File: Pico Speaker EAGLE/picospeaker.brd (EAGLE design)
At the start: 77.1 x 76.2 mm, 9 parts, among them J1 SPK -/+ MAX 3W, J2 POWER -/+ 4,5v

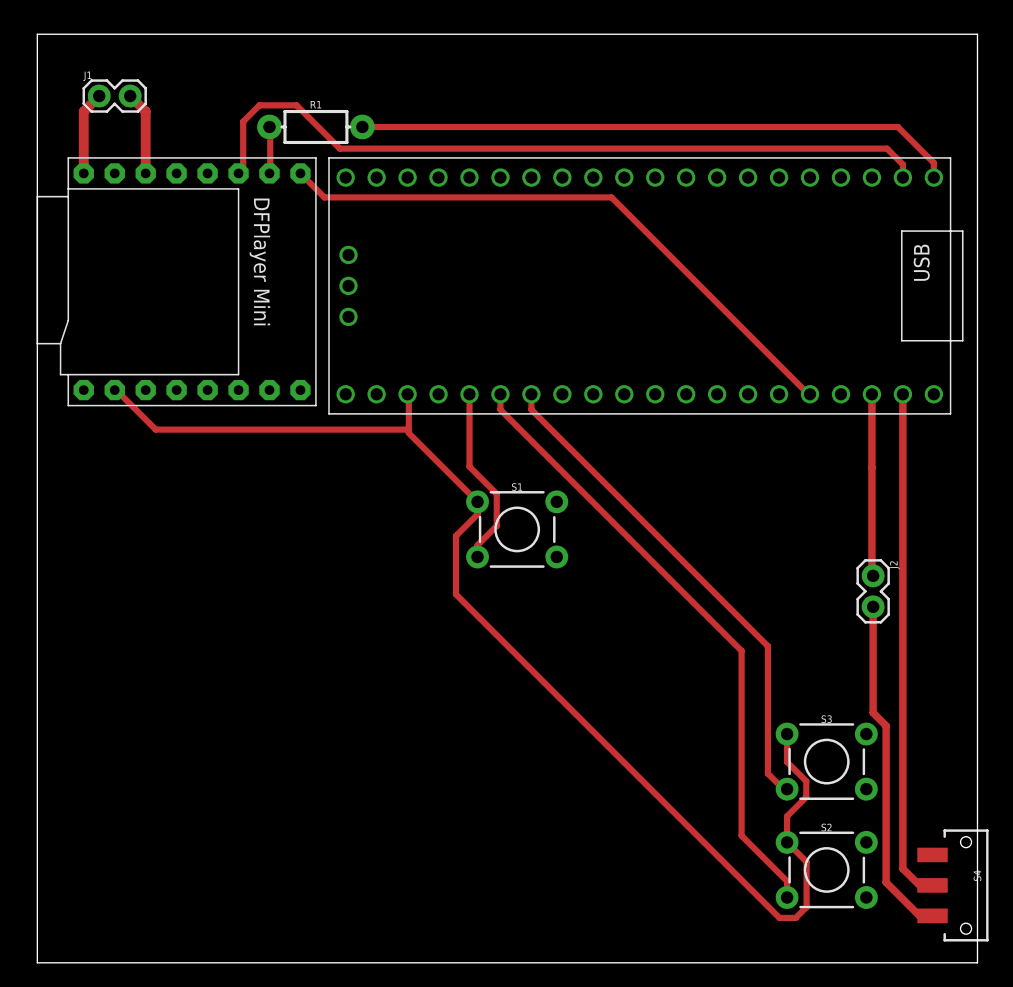
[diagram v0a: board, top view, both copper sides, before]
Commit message: Updates
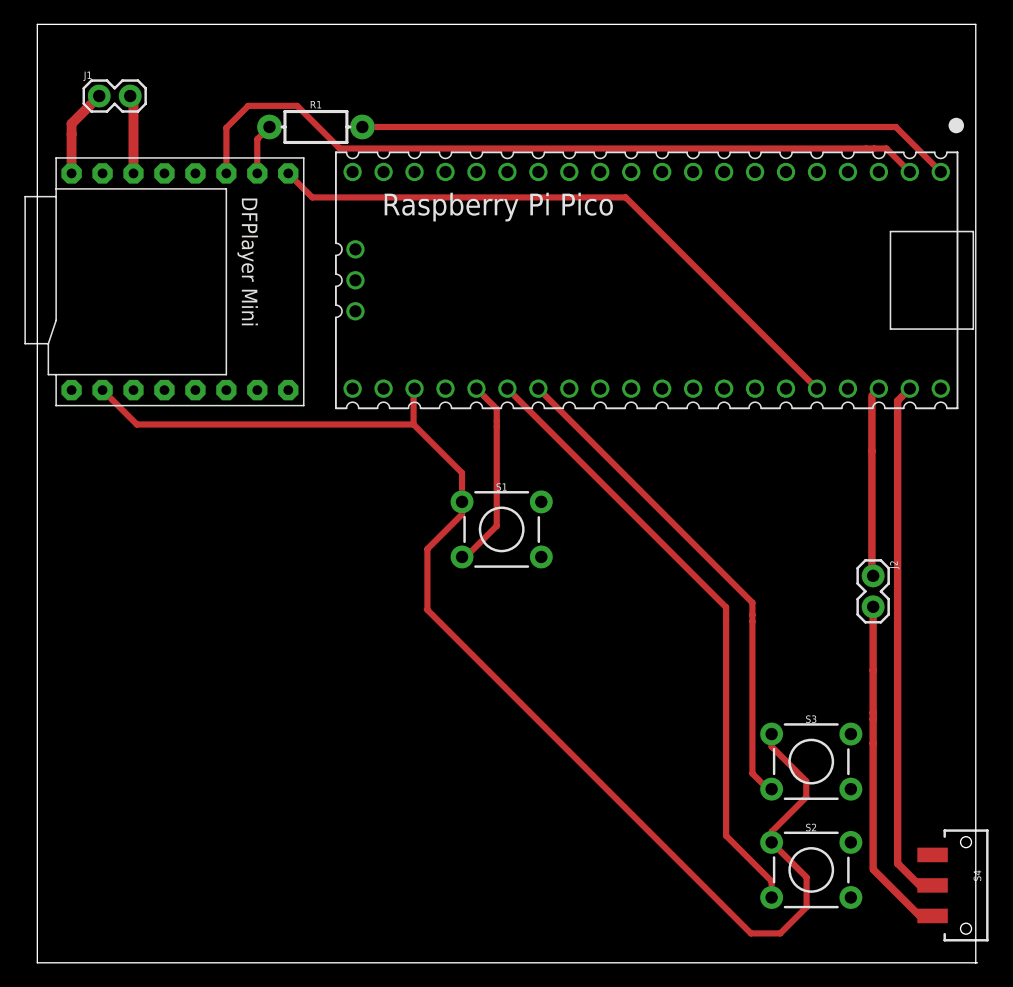
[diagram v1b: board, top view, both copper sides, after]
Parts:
- U$1: value RASPBERRY-PI-PICO_TH -> RASPBERRY-PI-PICO; device pipico:FT_RASPBERRY-PI-PICO_TH -> Proper-Pico:PICO-PKG-TH
- moved S1 1.27 mm to (38.1, 35.6)
- moved S2 1.27 mm to (63.5, 7.62)
- moved S3 1.27 mm to (63.5, 16.5)
- moved U$2 1.00 mm to (11.7, 55.9)
- moved U$1 0.49 mm to (50.0, 56.0)
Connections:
- new net GND1: U$1.3
- new net GND2: U$1.8
- new net GND3: U$1.13
- new net GND4: U$1.18
- new net GND6: U$1.28
- new net GND7: U$1.33
- new net GND9: U$1.42
- new net VBUS: U$1.40
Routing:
- net N$8: track 101.3 -> 108.5 mm
- net N$11: track 40.9 -> 43.0 mm
- net N$3: track 49.3 -> 50.7 mm
- net N$10: track 14.9 -> 15.9 mm
- net N$13: track 14.9 -> 15.6 mm
- net N$7: track 62.2 -> 62.8 mm
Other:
- board size 77.1 x 76.2 mm -> 77.1 x 77 mm
